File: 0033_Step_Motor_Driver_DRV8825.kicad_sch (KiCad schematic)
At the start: 9 parts, among them M1 DRV8825PWP

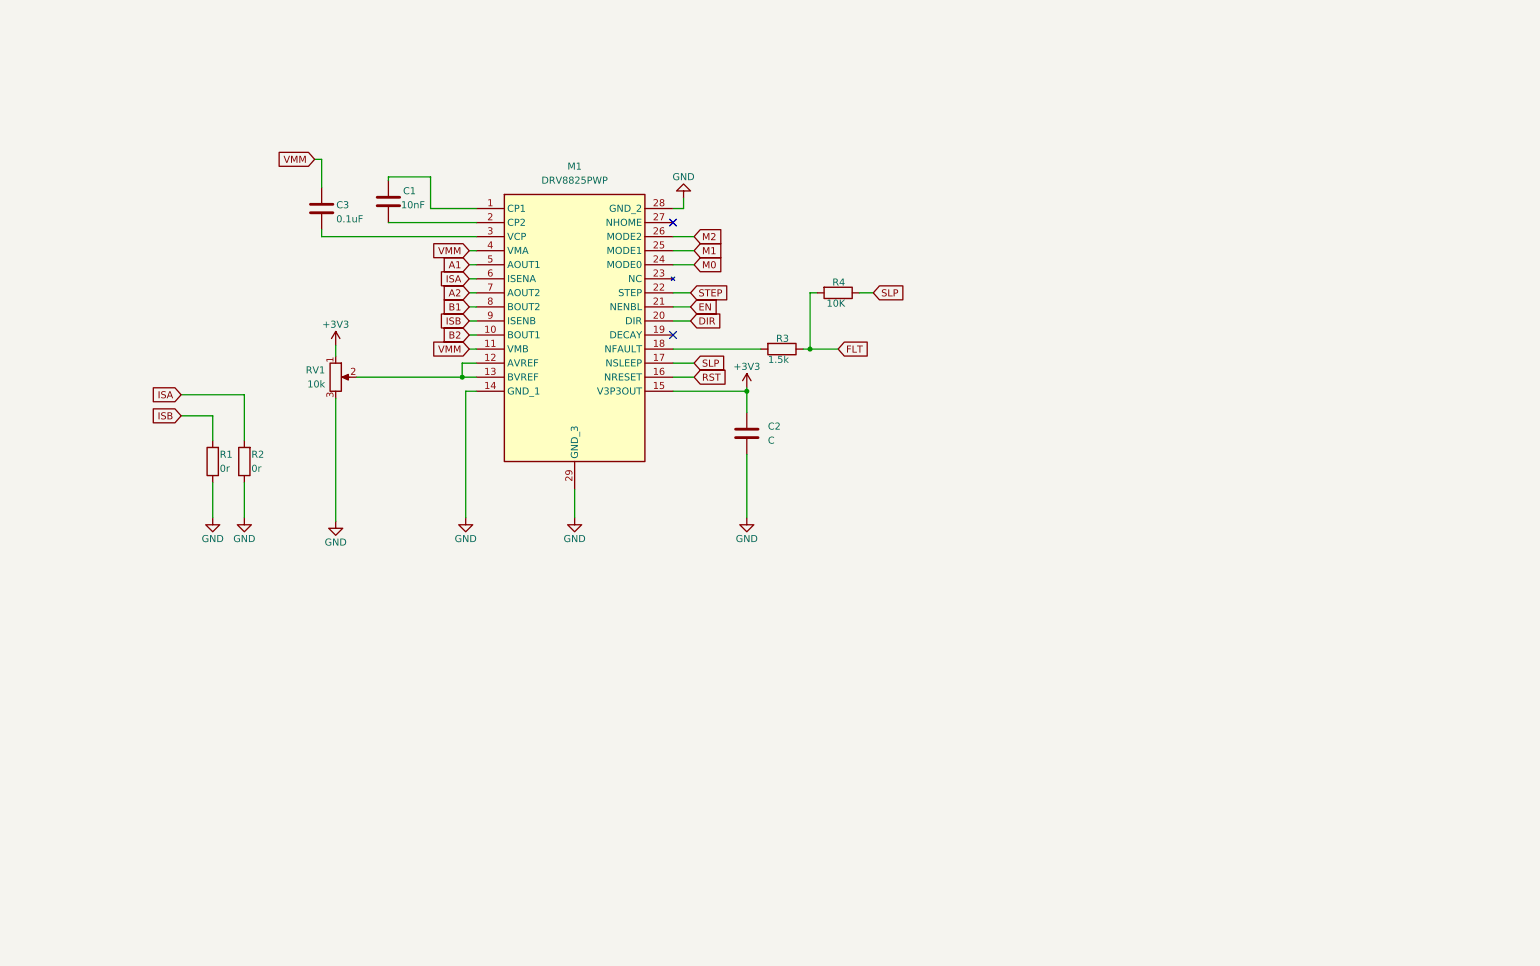
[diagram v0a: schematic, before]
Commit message: Add files via upload
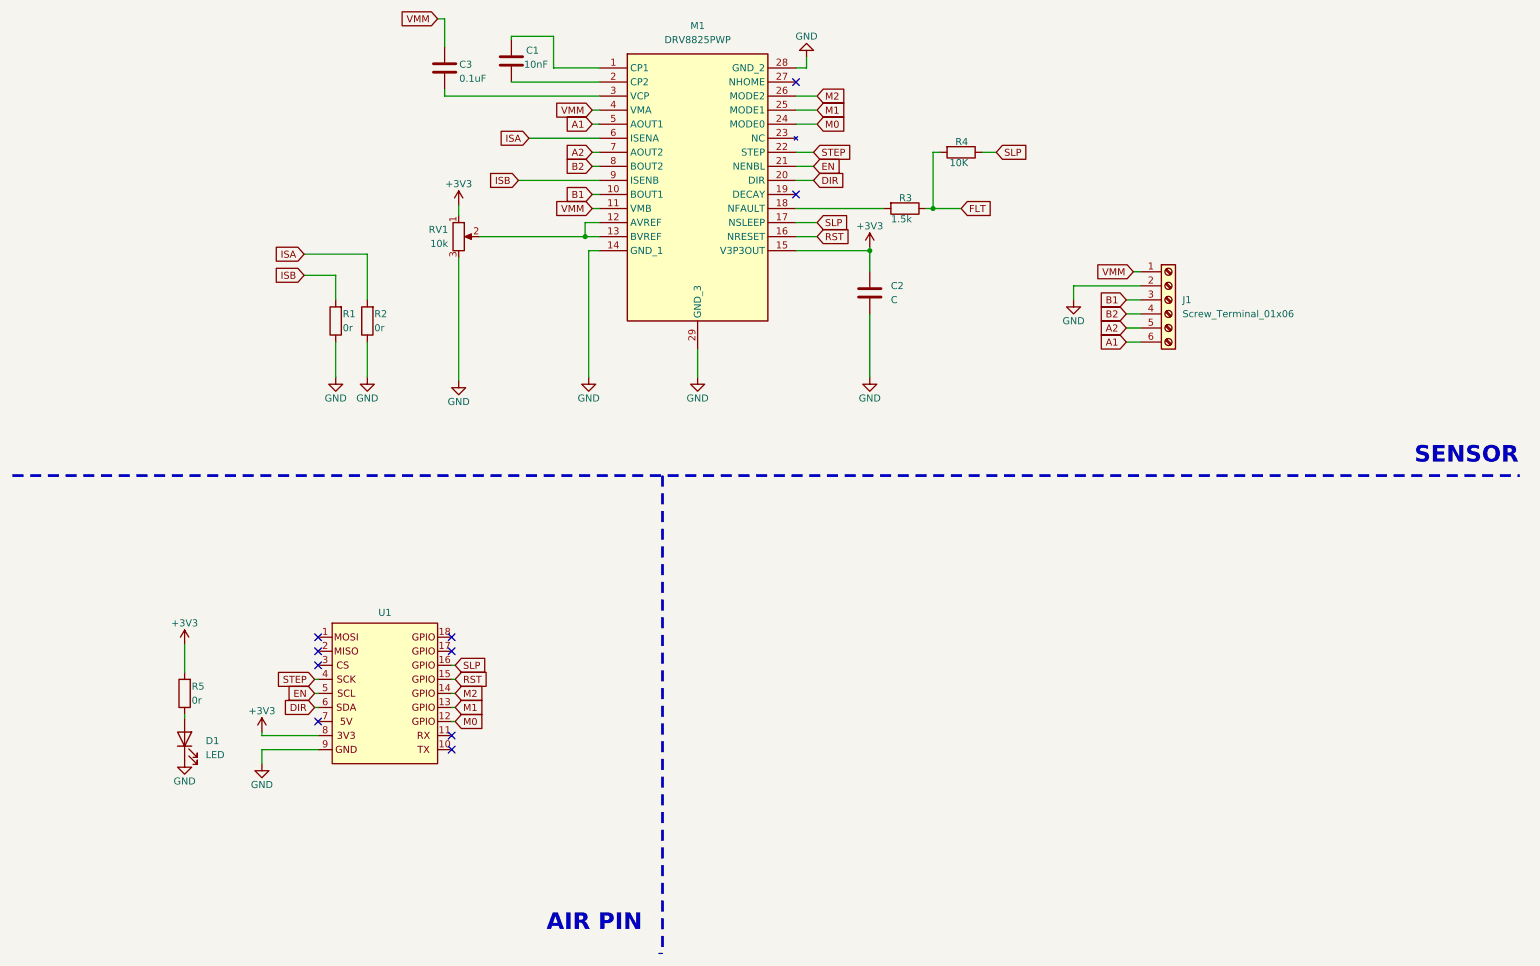
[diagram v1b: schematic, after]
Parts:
- added D1: LED, LED_SMD:LED_0805_2012Metric, symbol Device:LED
- added J1: Screw_Terminal_01x06, Connector_PinHeader_2.54mm:PinHeader_1x06_P2.54mm_Vertical, symbol Connector:Screw_Terminal_01x06
- added R5: 0r, Resistor_SMD:R_0603_1608Metric, symbol Device:R
- added U1: ~, Moduler_:pin_header, symbol moduler_pin:air
- C1, C2, C3: footprint (none) -> Capacitor_SMD:C_0603_1608Metric
- M1: footprint SOP65P640X120-29N -> DRV8825:SOP65P640X120-29N
- R1, R2, R3, R4: footprint (none) -> Resistor_SMD:R_0603_1608Metric
- RV1: footprint (none) -> memin:3362P_1
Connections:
- net +3V3: now also R5.2, U1.8
- net A1: now also J1.6 (Pin_6)
- net A2: now also J1.5 (Pin_5)
- net B1: now also M1.10 (BOUT1), J1.3 (Pin_3); no longer M1.8 (BOUT2)
- net B2: now also M1.8 (BOUT2), J1.4 (Pin_4); no longer M1.10 (BOUT1)
- net DIR: now also U1.6
- net EN: now also U1.5
- net GND: now also D1.1 (K), J1.2 (Pin_2), U1.9
- net M0: now also U1.12
- net M1: now also U1.13
- net M2: now also U1.14
- net RST: now also U1.15
- net SLP: now also U1.16
- net STEP: now also U1.4
- net VMM: now also J1.1 (Pin_1)
- new net: D1.2 (A), R5.1
- no-connect marks 2 -> 10
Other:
- note added: "AIR PIN"
- note added: "SENSOR"
- moved on the sheet: C1, C2, C3, M1, R1, R2, R3, R4, RV1
